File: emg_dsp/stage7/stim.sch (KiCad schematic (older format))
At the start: 7 parts

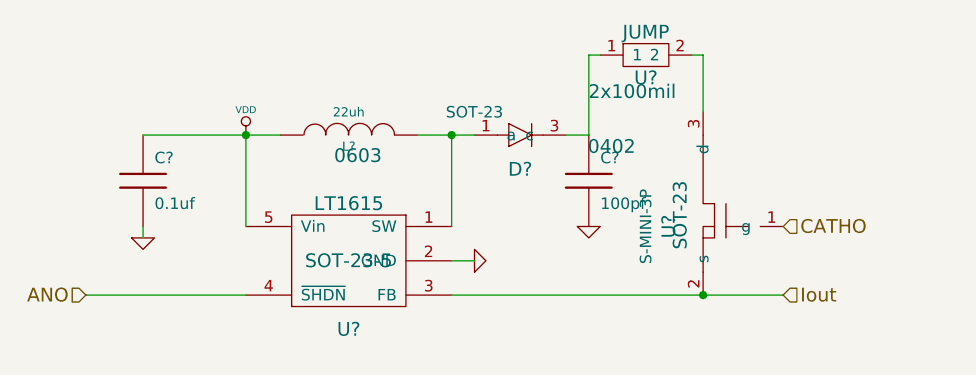
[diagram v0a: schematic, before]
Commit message: woooo working on the next microstimulator.
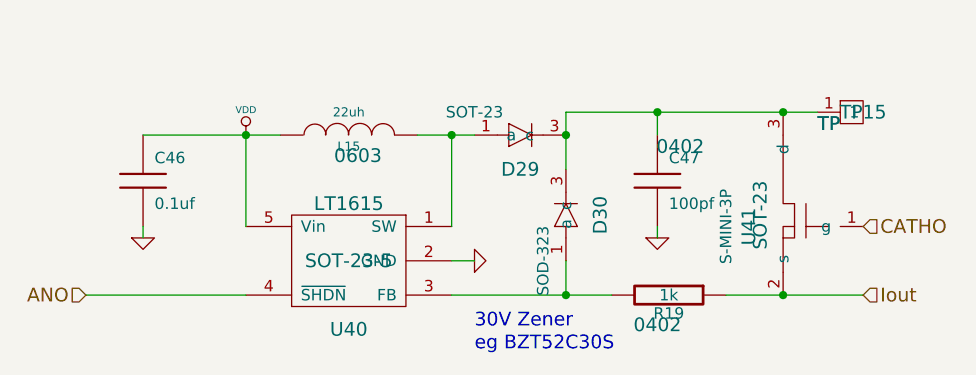
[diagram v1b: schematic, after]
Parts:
- removed U?: JUMP, 2x100mil, symbol JUMP
- added D2: D, SOD-323, symbol D
- added R5: 1k, 0402, symbol R
- added TP1: TP, TP, symbol TP
- gave numbers to parts that had none: 6
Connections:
- net Iout: now also R5.1; no longer U12.3 (FB)
- net at C19.1, D1.3 (c): now also U13.3 (d), D2.3 (c), TP1.1
- new net: D2.1 (a), R5.2, U12.3 (FB)
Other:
- note added: "30V Zener"
- note added: "eg BZT52C30S"
- moved on the sheet: C47, U41
